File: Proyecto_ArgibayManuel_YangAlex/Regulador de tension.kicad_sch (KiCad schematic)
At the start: 10 parts, among them IC1 LM1117

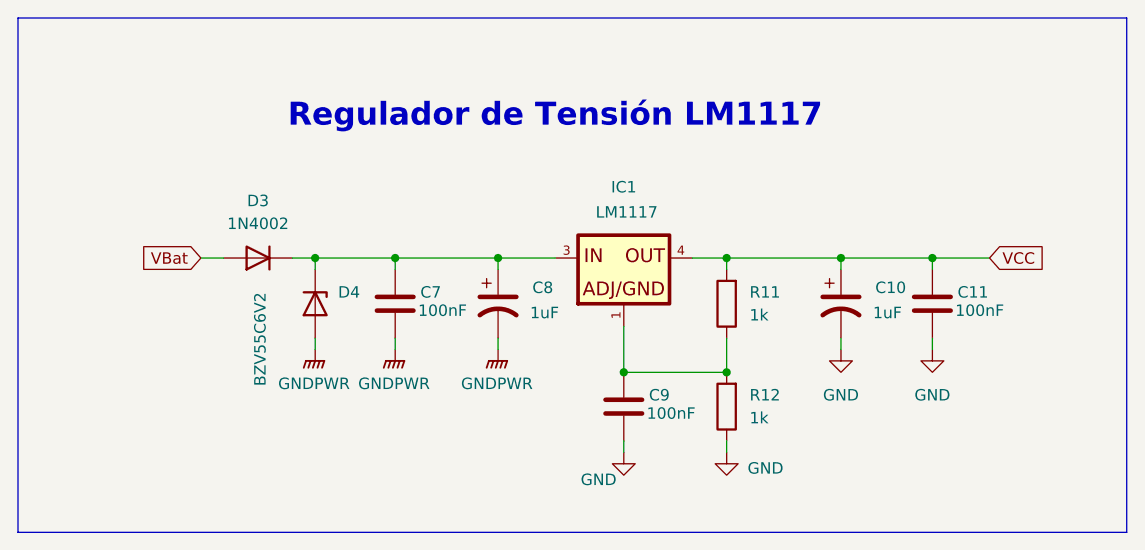
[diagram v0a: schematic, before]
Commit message: sensor
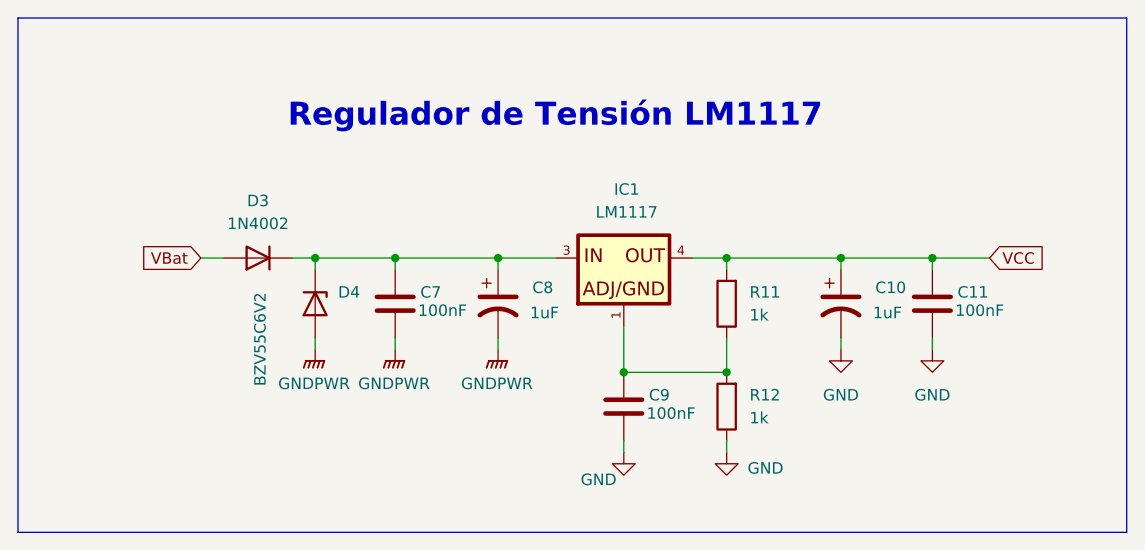
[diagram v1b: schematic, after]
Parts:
- C10, C11, C7, C8, C9: footprint (none) -> Capacitor_SMD:C_0805_2012Metric
- IC1: footprint (none) -> LM1117:SOT223
- R11, R12: footprint (none) -> Resistor_THT:R_Axial_DIN0204_L3.6mm_D1.6mm_P1.90mm_Vertical
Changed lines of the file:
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@@
+	)
+	(symbol
+		(lib_id "LM1117:LM1117")
+		(at 80.01 39.37 0)
+		(unit 1)
+		(exclude_from_sim no)
+		(in_bom yes)
+		(on_board yes)
+		(dnp no)
+		(fields_autoplaced yes)
+		(property "Reference" "IC1"
+			(at 80.3354 31.75 0)
+			(effects
+				(font
+					(size 1.27 1.27)
+				)
+			)
+		)
+		(property "Value" "LM1117"
+			(at 80.3354 34.29 0)
+			(effects
+				(font
+					(size 1.27 1.27)
+				)
+			)
+		)
+		(property "Footprint" "LM1117:SOT223"
+			(at 80.01 39.37 0)
+			(effects
+				(font
+					(size 1.27 1.27)
+				)
+				(hide yes)
+			)
+		)
+		(property "Datasheet" ""
+			(at 80.01 39.37 0)
+			(effects
+				(font
+					(size 1.27 1.27)
+				)
+				(hide yes)
+			)
+		)
+		(property "Description" ""
+			(at 80.01 39.37 0)
+			(effects
+				(font
+					(size 1.27 1.27)
+				)
+				(hide yes)
+			)
+		)
+		(property "MF" "Texas Instruments"
+			(at 80.01 39.37 0)
+			(effects
+				(font
+					(size 1.27 1.27)
+				)
+				(justify bottom)
+				(hide yes)
+			)
+		)
+		(property "Description_1" "1A Low Dropout Positive Voltage Regulator"
+			(at 80.01 39.37 0)
+			(effects
+				(font
+					(size 1.27 1.27)
+				)
+				(justify bottom)
+				(hide yes)
+			)
+		)
+		(property "Package" "None"
+			(at 80.01 39.37 0)
+			(effects
+				(font
+					(size 1.27 1.27)
+				)
+				(justify bottom)
+				(hide yes)
+			)
+		)
+		(property "Price" "None"
+			(at 80.01 39.37 0)
+			(effects
+				(font
+					(size 1.27 1.27)
+				)
+				(justify bottom)
+				(hide yes)
+			)
+		)
+		(property "SnapEDA_Link" "https://www.snapeda.com/parts/LM1117/Texas+Instruments/view-part/?ref=snap"
+			(at 80.01 39.37 0)
+			(effects
+				(font
+					(size 1.27 1.27)
+				)
+				(justify bottom)
+				(hide yes)
+			)
+		)
+		(property "MP" "LM1117"
+			(at 80.01 39.37 0)
+			(effects
+				(font
+					(size 1.27 1.27)
+				)
+				(justify bottom)
+				(hide yes)
+			)
+		)
+		(property "Availability" "Not in stock"
+			(at 80.01 39.37 0)
+			(effects
+				(font
+					(size 1.27 1.27)
+				)
+				(justify bottom)
+				(hide yes)
+			)
+		)
+		(property "Check_prices" "https://www.snapeda.com/parts/LM1117/Texas+Instruments/view-part/?ref=eda"
+			(at 80.01 39.37 0)
+			(effects
+				(font
+					(size 1.27 1.27)
+				)
+				(justify bottom)
+				(hide yes)
+			)
+		)
+		(pin "1"
+		)
+		(pin "3"
+		)
+		(pin "4"
+		)
+		(instances
+			(project ""
+				(path "/b2dde924-33f5-41ab-a1bf-811873450a89/586cebd2-39d7-435a-989d-0b17f5522a13"
+					(reference "IC1")
+					(unit 1)
+				)
+			)
+		)
 	)
 	(symbol
@@
 			)
 		)
-		(property "Footprint" ""
+		(property "Footprint" "Capacitor_SMD:C_0805_2012Metric"
 			(at 55.5752 48.26 0)
 			(effects
@@
 	)
 	(symbol
-		(lib_id "LM1117:LM1117")
-		(at 80.01 39.37 0)
-		(unit 1)
-		(exclude_from_sim no)
-		(in_bom yes)
-		(on_board yes)
-		(dnp no)
-		(property "Reference" "IC1"
-			(at 80.01 31.496 0)
-			(effects
-				(font
-					(size 1.27 1.27)
-				)
-			)
-		)
-		(property "Value" "LM1117"
-			(at 80.3354 34.29 0)
-			(effects
-				(font
-					(size 1.27 1.27)
-				)
-			)
-		)
-		(property "Footprint" ""
-			(at 80.01 39.37 0)
-			(effects
-				(font
-					(size 1.27 1.27)
-				)
-				(hide yes)
-			)
-		)
-		(property "Datasheet" ""
-			(at 80.01 39.37 0)
-			(effects
-				(font
-					(size 1.27 1.27)
-				)
-				(hide yes)
-			)
-		)
-		(property "Description" ""
-			(at 80.01 39.37 0)
-			(effects
-				(font
-					(size 1.27 1.27)
-				)
-				(hide yes)
-			)
-		)
-		(property "MF" "Texas Instruments"
-			(at 80.01 39.37 0)
-			(effects
-				(font
-					(size 1.27 1.27)
-				)
-				(justify bottom)
-				(hide yes)
-			)
-		)
-		(property "Description_1" "1A Low Dropout Positive Voltage Regulator"
-			(at 80.01 39.37 0)
-			(effects
-				(font
-					(size 1.27 1.27)
-				)
-				(justify bottom)
-				(hide yes)
-			)
-		)
-		(property "Package" "None"
-			(at 80.01 39.37 0)
-			(effects
-				(font
-					(size 1.27 1.27)
-				)
-				(justify bottom)
-				(hide yes)
-			)
-		)
-		(property "Price" "None"
-			(at 80.01 39.37 0)
-			(effects
-				(font
-					(size 1.27 1.27)
-				)
-				(justify bottom)
-				(hide yes)
-			)
-		)
-		(property "SnapEDA_Link" "https://www.snapeda.com/parts/LM1117/Texas+Instruments/view-part/?ref=snap"
-			(at 80.01 39.37 0)
-			(effects
-				(font
-					(size 1.27 1.27)
-				)
-				(justify bottom)
-				(hide yes)
-			)
-		)
-		(property "MP" "LM1117"
-			(at 80.01 39.37 0)
-			(effects
-				(font
-					(size 1.27 1.27)
-				)
-				(justify bottom)
-				(hide yes)
-			)
-		)
-		(property "Availability" "Not in stock"
-			(at 80.01 39.37 0)
-			(effects
-				(font
-					(size 1.27 1.27)
-				)
-				(justify bottom)
-				(hide yes)
-			)
-		)
-		(property "Check_prices" "https://www.snapeda.com/parts/LM1117/Texas+Instruments/view-part/?ref=eda"
-			(at 80.01 39.37 0)
-			(effects
-				(font
-					(size 1.27 1.27)
-				)
-				(justify bottom)
-				(hide yes)
-			)
-		)
-		(pin "4"
-		)
-		(pin "3"
-		)
-		(pin "1"
-		)
-		(instances
-			(project "Proyecto_ArgibayManuel_YangAlex"
-				(path "/b2dde924-33f5-41ab-a1bf-811873450a89/586cebd2-39d7-435a-989d-0b17f5522a13"
-					(reference "IC1")
-					(unit 1)
-				)
-			)
-		)
-	)
-	(symbol
 		(lib_id "Device:C_Polarized_US")
 		(at 66.04 44.45 0)
@@
 			)
 		)
-		(property "Footprint" ""
+		(property "Footprint" "Capacitor_SMD:C_0805_2012Metric"
 			(at 66.04 44.45 0)
 			(effects
@@
 			)
 		)
-		(property "Footprint" ""
+		(property "Footprint" "Resistor_THT:R_Axial_DIN0204_L3.6mm_D1.6mm_P1.90mm_Vertical"
 			(at 93.218 44.45 90)
 			(effects
@@
 			)
 		)
-		(property "Footprint" ""
+		(property "Footprint" "Resistor_THT:R_Axial_DIN0204_L3.6mm_D1.6mm_P1.90mm_Vertical"
 			(at 93.218 55.88 90)
 			(effects
@@
 			)
 		)
-		(property "Footprint" ""
+		(property "Footprint" "Capacitor_SMD:C_0805_2012Metric"
 			(at 80.9752 59.69 0)
 			(effects
@@
 			)
 		)
-		(property "Footprint" ""
+		(property "Footprint" "Capacitor_SMD:C_0805_2012Metric"
 			(at 115.2652 48.26 0)
 			(effects
@@
 			)
 		)
-		(property "Footprint" ""
+		(property "Footprint" "Capacitor_SMD:C_0805_2012Metric"
 			(at 104.14 44.45 0)
 			(effects
